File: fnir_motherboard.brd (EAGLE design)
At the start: 33.6 x 43.5 mm, 44 parts, among them IC1 LTC2494, IC3 AD712R, U2 ATMEGA8U2QFN, X2 USB-SMD-NS, Y1 16MHz

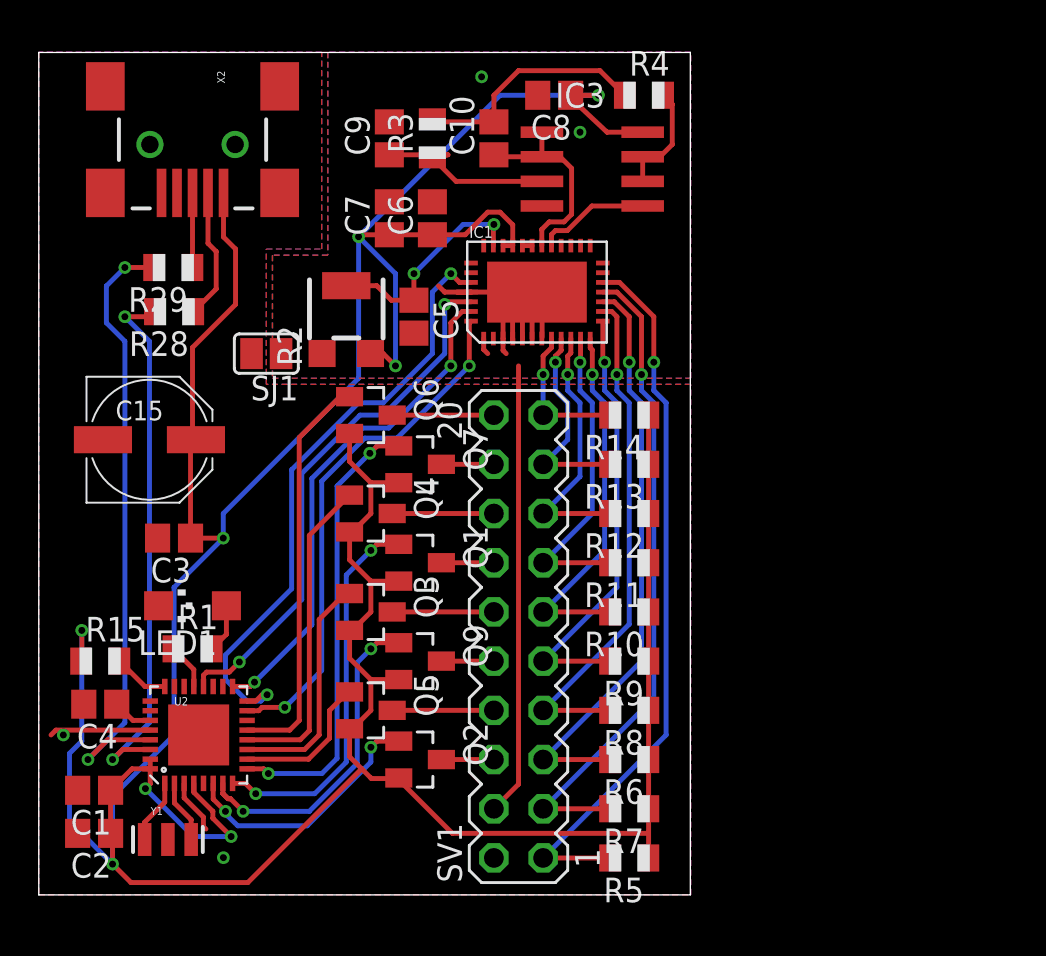
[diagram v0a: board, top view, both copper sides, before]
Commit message: new version desinged
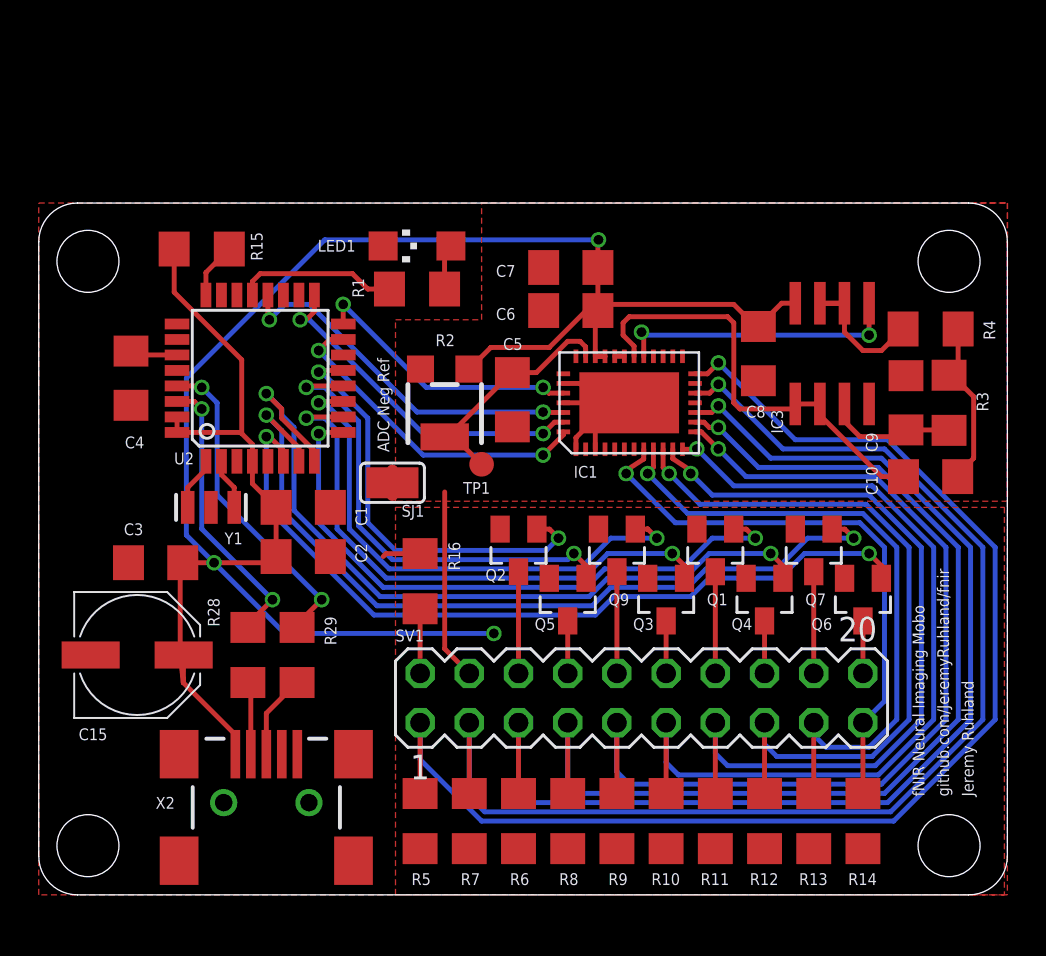
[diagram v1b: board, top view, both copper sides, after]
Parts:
- added R16: 200, adafruit:R1206
- added TP1: PTR1B1,27, testpad:B1,27
- C1, C2, C3, C4, C5, C6, C7, C8: device adafruit:C0805 -> adafruit:C1206
- C10, C9: value (none) -> 0.1uF; device adafruit:C0805 -> adafruit:C1206
- R1: value (none) -> 200; device adafruit:R0805 -> adafruit:R1206
- R10, R11, R12, R13, R14, R15, R28, R29, R5, R6, R7, R8, R9: device adafruit:R0805 -> adafruit:R1206
- R2: value (none) -> 10k
- R3, R4: value (none) -> 30k; device adafruit:R0805 -> adafruit:R1206
- U2: value ATMEGA8U2QFN -> ATMEGA8U2AU; device sparkfun:QFN-32 -> sparkfun:TQFP32-08
- moved X2 34.2 mm to (11.7, 4.76), turned to 90 degrees
- moved R3 30.0 mm to (47.0, 25.4)
- moved C9 30.0 mm to (44.8, 25.4)
- moved C10 28.5 mm to (46.0, 21.6), turned to 0 degrees
- moved Q6 27.1 mm to (42.5, 15.2), turned to 180 degrees
- moved R14 24.2 mm to (42.5, 3.81), turned to 90 degrees
- moved R15 21.9 mm to (8.41, 33.3)
- moved LED1 21.9 mm to (19.5, 33.5)
- moved R1 21.9 mm to (19.5, 31.3)
- moved R29 21.0 mm to (13.3, 12.4), turned to 90 degrees
- moved Q4 20.8 mm to (37.5, 15.2), turned to 180 degrees
- moved Q7 20.8 mm to (40.0, 17.8), turned to 180 degrees
- moved R13 20.7 mm to (40.0, 3.81), turned to 90 degrees
- moved R4 19.1 mm to (46.0, 29.2), turned to 180 degrees
- moved U2 18.7 mm to (11.4, 26.7), turned to 90 degrees
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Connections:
- new net N$23: R16.2, SV1.2
- net +5V: now also R2.1; no longer R2.3
- net AGND: now also R2.3; no longer R2.1
- net GND: now also R16.1; no longer SV1.2
- net IR8: now also IC1.17; no longer IC1.16
- net IR9: now also IC1.19; no longer IC1.17
- net N$1: now also Q2.1; no longer Q6.1
- net N$12: now also TP1.TP
- net N$2: now also Q1.1; no longer Q7.1
- net N$3: now also Q9.1, U2.11; no longer Q5.1, U2.10
- net N$4: now also Q4.1; no longer Q1.1
- net N$5: now also Q5.1; no longer Q4.1
- net N$6: now also Q7.1; no longer Q9.1
- net N$7: now also Q6.1; no longer Q2.1
- net N$8: now also U2.10; no longer U2.11
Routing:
- net +5V: track 212.0 -> 116.5 mm, vias 8 -> 3
- net IR8: track 34.0 -> 63.7 mm
- net IR9: track 37.6 -> 67.3 mm
- net IR7: track 30.4 -> 58.8 mm
- net N$7: track 13.3 -> 41.7 mm
- net IR6: track 26.7 -> 53.8 mm
- net IR5: track 22.9 -> 49.1 mm
- net IR4: track 19.2 -> 44.9 mm
- net N$6: track 17.1 -> 42.7 mm
- net IR3: track 16.3 -> 41.3 mm
- net IR2: track 13.6 -> 37.5 mm
- net IR1: track 10.8 -> 34.1 mm
- net IR0: track 7.57 -> 29.8 mm
- net N$4: track 19.8 -> 40.1 mm
- net N$3: track 7.57 -> 27.4 mm, vias 0 -> 2
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- added copper zone on layer 1, net +5V
- removed copper zone on layer 16, net AGND
- removed copper zone on layer 16, net GND
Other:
- board size 33.6 x 43.5 mm -> 50 x 35.7 mm
- board text added: "ADC Neg Ref"
- board text added: "Jeremy Ruhland"
- board text added: "fNIR Neural Imaging Mobo"
- board text added: "github.com/JeremyRuhland/fnir"
